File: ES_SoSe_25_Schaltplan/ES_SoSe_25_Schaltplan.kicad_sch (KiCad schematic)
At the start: 3 parts

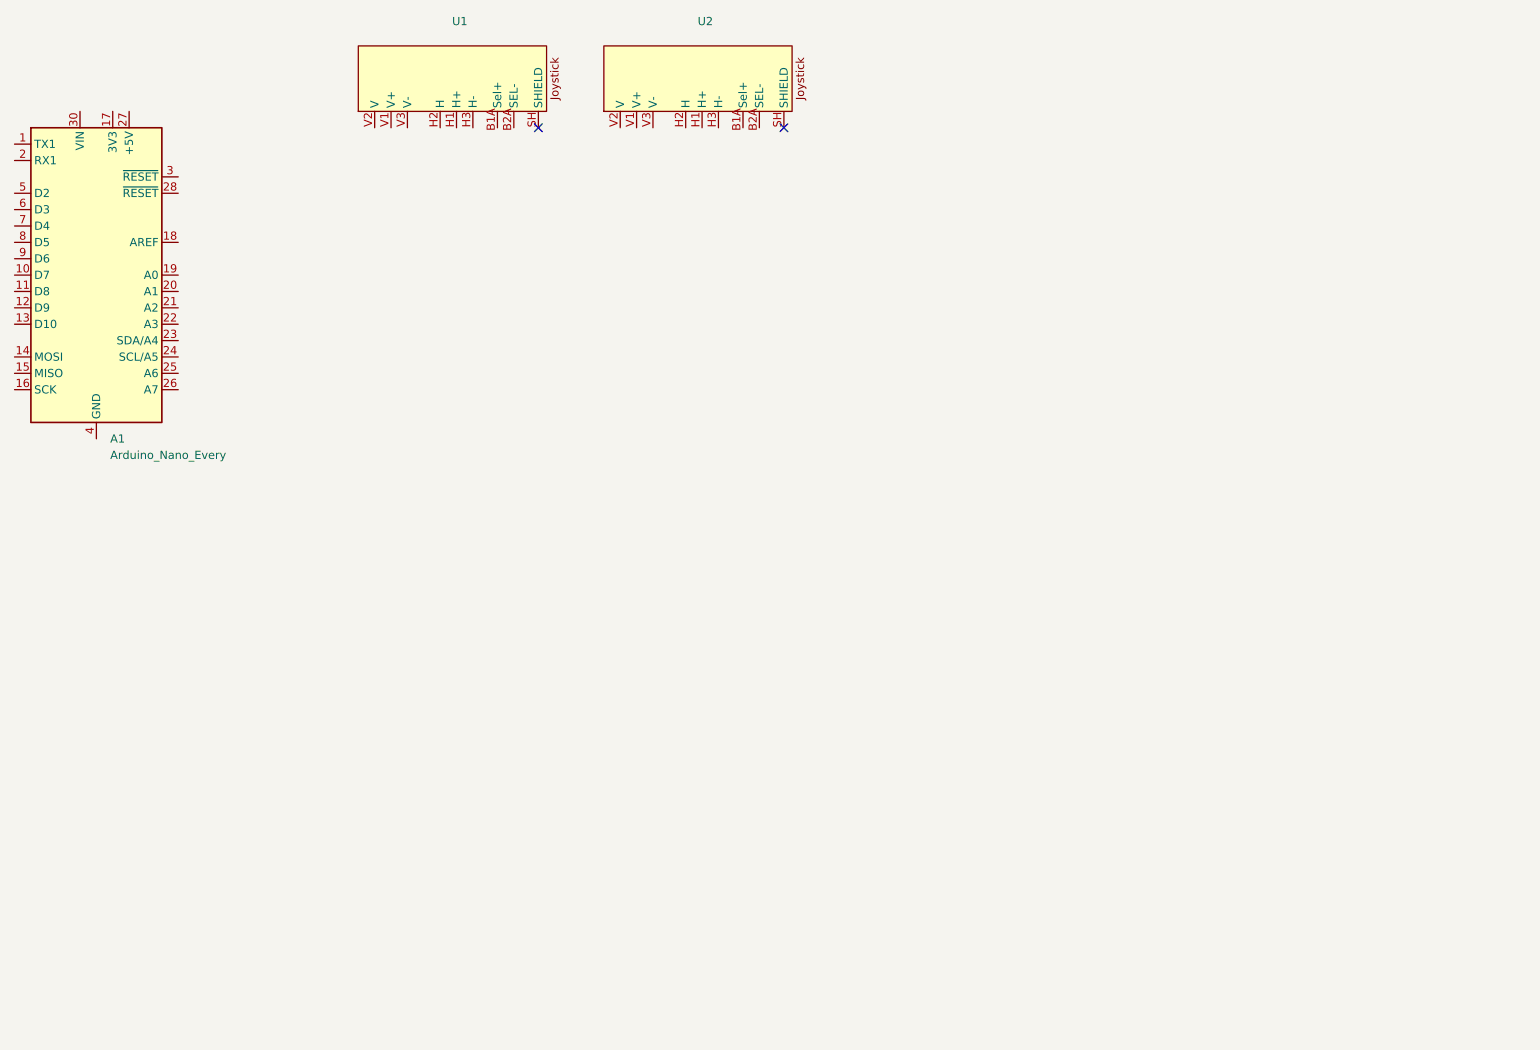
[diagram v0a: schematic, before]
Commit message: updated scematic
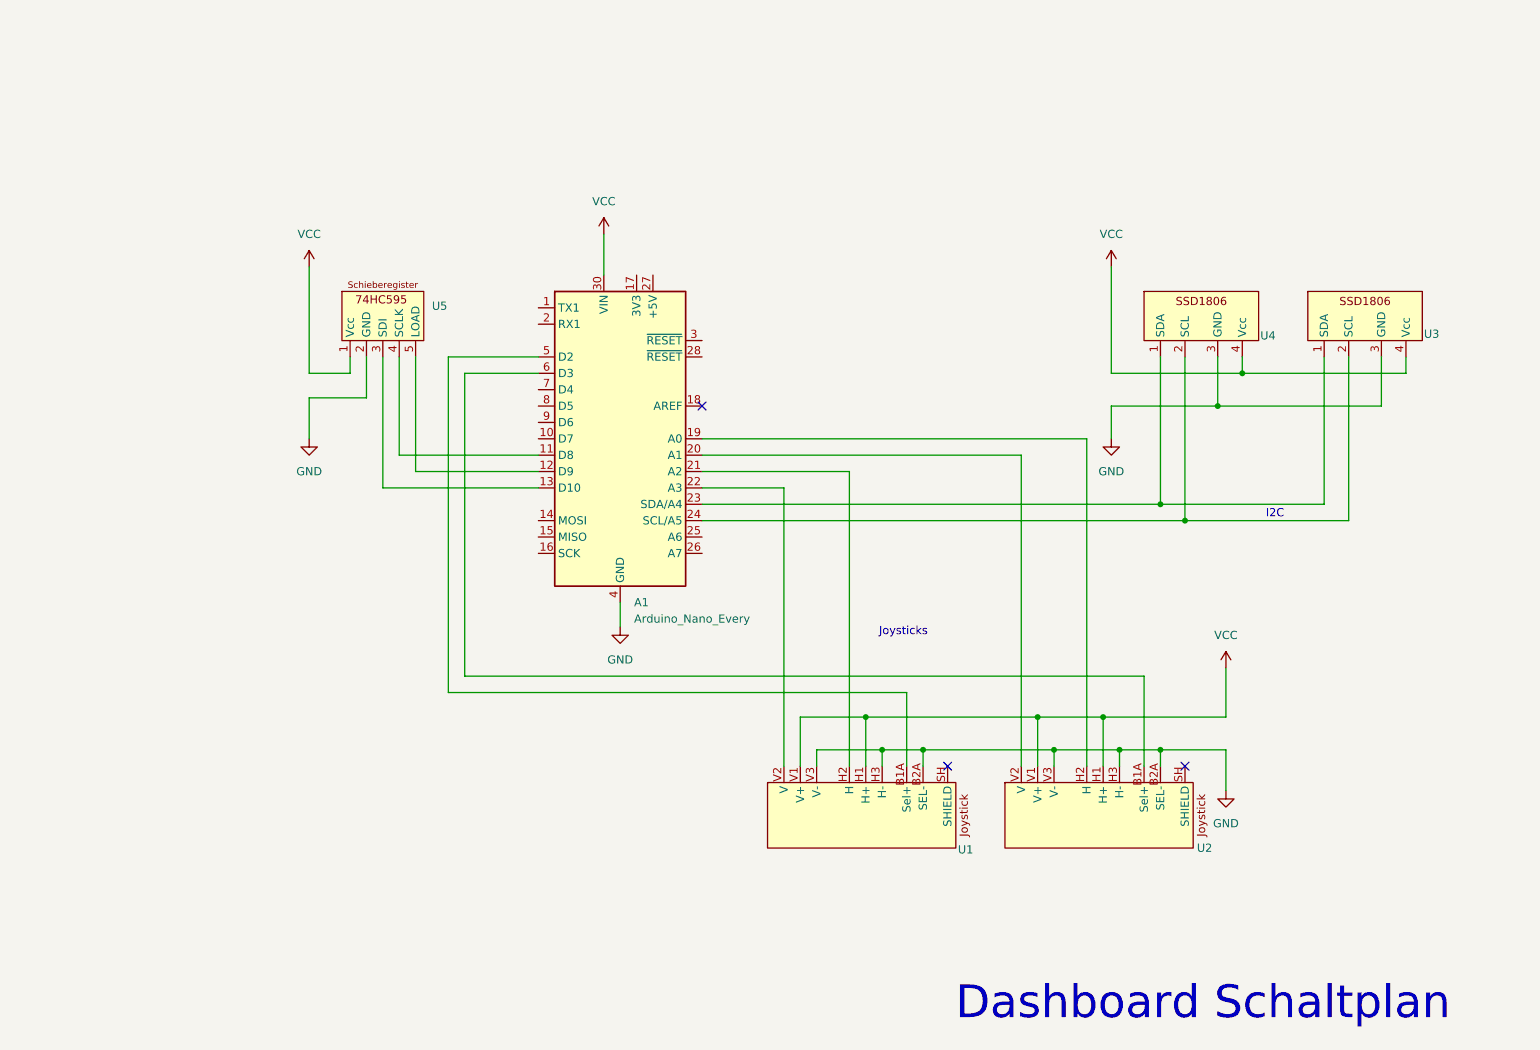
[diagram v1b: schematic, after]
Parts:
- added U3, U4: ~, symbol es_custom_symbols:SSD1806
- added U5: ~, symbol es_custom_symbols:74HC595
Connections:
- net at A1.11 (D8): now also U5.4 (SCLK)
- net at A1.12 (D9): now also U5.5 (LOAD)
- net at A1.13 (D10): now also U5.3 (SDI)
- net at A1.19 (A0): now also U2.H2 (H)
- net at A1.20 (A1): now also U2.V2 (V)
- net at A1.21 (A2): now also U1.H2 (H)
- net at A1.22 (A3): now also U1.V2 (V)
- net at A1.23 (SDA/A4): now also U3.1 (SDA), U4.1 (SDA)
- net at A1.24 (SCL/A5): now also U3.2 (SCL), U4.2 (SCL)
- net GND: now reaches A1.29 (GND), A1.4 (GND)
- net GND: now also U1.B2A (SEL-), U1.H3 (H-), U1.V3 (V-), U2.B2A (SEL-), U2.H3 (H-), U2.V3 (V-), U3.3 (GND), U4.3 (GND), U5.2 (GND)
- net VCC: now reaches A1.30 (VIN)
- net VCC: now also U1.H1 (H+), U1.V1 (V+), U2.H1 (H+), U2.V1 (V+), U3.4 (Vcc), U4.4 (Vcc), U5.1 (Vcc)
- net at A1.5 (D2): now also U1.B1A (Sel+)
- net at A1.6 (D3): now also U2.B1A (Sel+)
- no-connect marks 2 -> 3
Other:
- note added: "Dashboard Schaltplan"
- note added: "I2C"
- note added: "Joysticks"
- moved on the sheet: A1, U1, U2
